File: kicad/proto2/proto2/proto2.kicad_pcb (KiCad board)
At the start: 2 copper layers, 100 x 100 mm, 0 parts

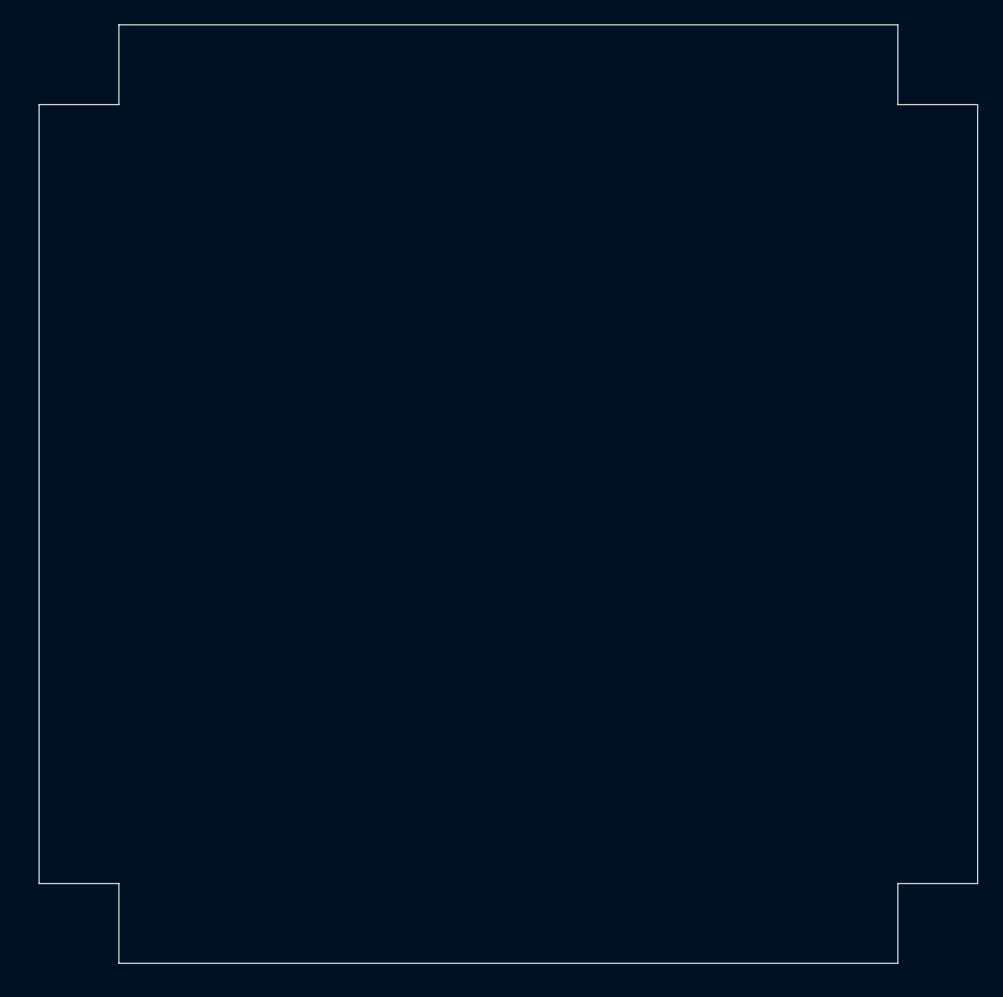
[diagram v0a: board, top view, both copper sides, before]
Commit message: pdf et png proto2
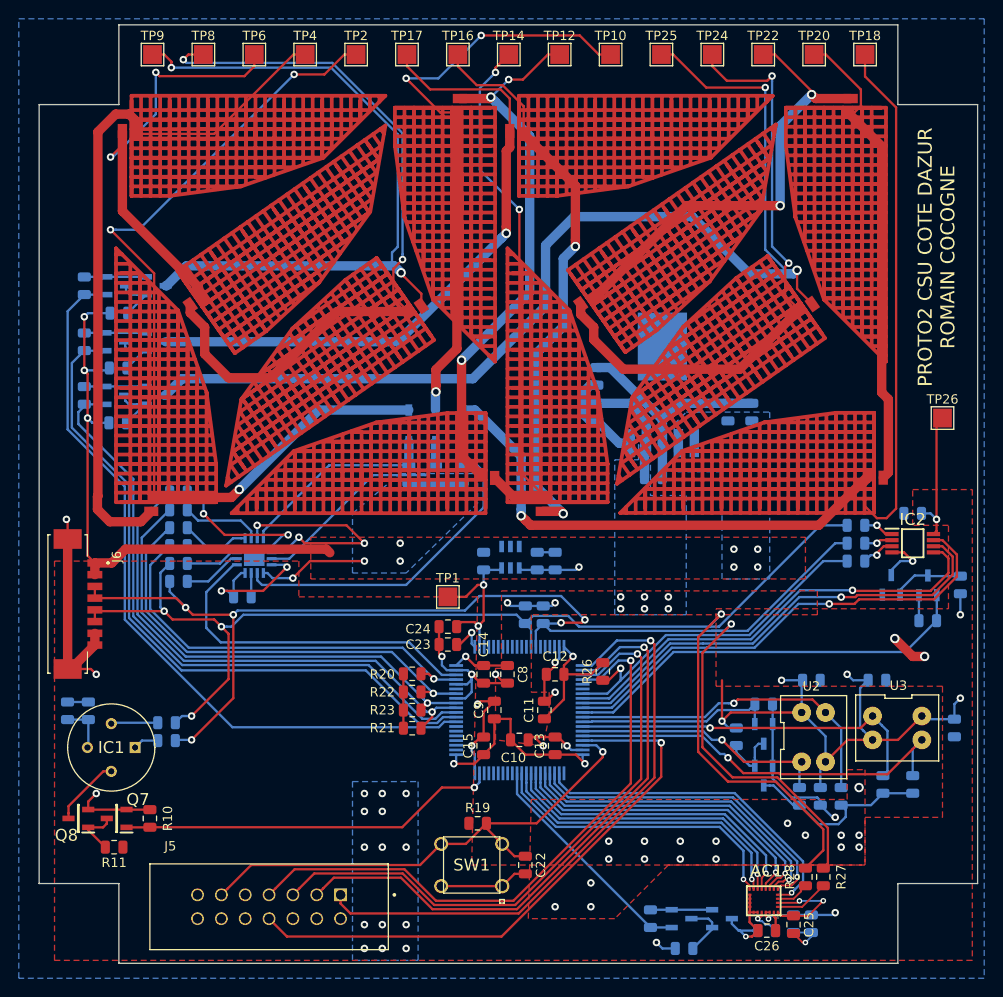
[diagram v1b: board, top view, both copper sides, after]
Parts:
- added AC1: LSM9DS1TR, panneaux_solaires:LGA-24L_3X3.5X1MM_, F.Cu at (168.3, 144.8)
- added C1: 100nF, Capacitor_SMD:C_0805_2012Metric, B.Cu at (144.1, 108.6)
- added C10: 10uF, Capacitor_SMD:C_0805_2012Metric, F.Cu at (142.2, 127.6)
- added C11: 10uF, Capacitor_SMD:C_0805_2012Metric, F.Cu at (144.9, 124.5)
- added C12: 10nF, Capacitor_SMD:C_0805_2012Metric, F.Cu at (146.1, 120.7)
- added C13: 10nF, Capacitor_SMD:C_0805_2012Metric, F.Cu at (146.1, 128.3)
- added C14: 10nF, Capacitor_SMD:C_0805_2012Metric, F.Cu at (138.4, 120.7)
- added C15: 10nF, Capacitor_SMD:C_0805_2012Metric, F.Cu at (138.4, 128.3)
- added C2: 1uF, Capacitor_SMD:C_0805_2012Metric, B.Cu at (146.1, 108.6)
- added C22: 2.2nF, Capacitor_SMD:C_0805_2012Metric, F.Cu at (142.9, 141.0)
- added C23: 100nF, Capacitor_SMD:C_0805_2012Metric, F.Cu at (134.6, 115.6)
- added C24: 100nF, Capacitor_SMD:C_0805_2012Metric, F.Cu at (134.6, 117.5)
- added C25: 100nF, Capacitor_SMD:C_0805_2012Metric, F.Cu at (171.4, 147.3)
- added C26: 100nF, Capacitor_SMD:C_0805_2012Metric, F.Cu at (168.6, 148.0)
- added C27: 10nF, Capacitor_SMD:C_0805_2012Metric, B.Cu at (168.6, 148.0)
- added C28: 100nF, Capacitor_SMD:C_0805_2012Metric, B.Cu at (173.4, 147.2)
- added C29: 10uF, Capacitor_SMD:C_0805_2012Metric, B.Cu at (171.4, 147.2)
- added C3: 1uF, Capacitor_SMD:C_0805_2012Metric, B.Cu at (138.4, 108.6)
- added C30: 100nF, Capacitor_SMD:C_0805_2012Metric, B.Cu at (174.3, 133.7)
- added C31: 100nF, Capacitor_SMD:C_0805_2012Metric, B.Cu at (180.3, 121.3)
- added C32: 100nF, Capacitor_SMD:C_0805_2012Metric, B.Cu at (188.6, 126.4)
- added C33: 100nF, Capacitor_SMD:C_0805_2012Metric, B.Cu at (173.4, 121.3)
- added C34: 100nF, Capacitor_SMD:C_0805_2012Metric, B.Cu at (164.5, 92.7)
- added C35: 2.2uF, Capacitor_SMD:C_0805_2012Metric, B.Cu at (167.0, 92.7)
- added C36: 47nF, Capacitor_SMD:C_0805_2012Metric, B.Cu at (156.5, 99.7)
- added C37: 100nF, Capacitor_SMD:C_0805_2012Metric, B.Cu at (112.7, 112.4)
- added C4: 10uF, Capacitor_SMD:C_0805_2012Metric, B.Cu at (96.3, 124.5)
- added C5: 100nF, Capacitor_SMD:C_0805_2012Metric, B.Cu at (94.1, 124.5)
- added C7: 100nF, Capacitor_SMD:C_0805_2012Metric, B.Cu at (184.2, 103.5)
- added C8: 10uF, Capacitor_SMD:C_0805_2012Metric, F.Cu at (141.0, 120.7)
- added C9: 10uF, Capacitor_SMD:C_0805_2012Metric, F.Cu at (139.6, 124.5)
- added D1: D_Schottky, panneaux_solaires:SOD3715X135N, B.Cu at (130.5, 94.2)
- added D2: D_Schottky, panneaux_solaires:SOD3715X135N, B.Cu at (133.3, 94.2)
- added D3: D_Schottky, panneaux_solaires:SOD3715X135N, B.Cu at (136.1, 94.2)
- added IC1: MLX90641ESF-BAA-000-TU, panneaux_solaires:MLX90621ESFBAB000SP, F.Cu at (101.3, 128.4)
- added IC2: PCT2075DP,118, panneaux_solaires:SOP65P490X110-8N, F.Cu at (184.2, 106.7)
- added IC3: MSP430FR5964IPNR, panneaux_solaires:QFP50P1400X1400X160-80N, B.Cu at (142.2, 124.5)
- added J5: HEADER_2x7_2.54MM, panneaux_solaires:TE_5104338-2, F.Cu at (123.2, 144.1)
- added J6: 0532610871, panneaux_solaires:MOLEX_0532610871, F.Cu at (94.1, 113.2)
- added Q1: RUR040N02HZGTL, panneaux_solaires:RUR040N02HZGTL, B.Cu at (99.3, 79.2)
- added Q10: RUR040N02HZGTL, panneaux_solaires:RUR040N02HZGTL, B.Cu at (181.9, 111.1)
- added Q11: RUR040N02HZGTL, panneaux_solaires:RUR040N02HZGTL, B.Cu at (159.5, 146.7)
- added Q12: RUR040N02HZGTL, panneaux_solaires:RUR040N02HZGTL, B.Cu at (163.8, 146.7)
- added Q13: RUR040N02HZGTL, panneaux_solaires:RUR040N02HZGTL, B.Cu at (168.3, 127.0)
- added Q14: RUR040N02HZGTL, panneaux_solaires:RUR040N02HZGTL, B.Cu at (168.3, 131.4)
- added Q2: RUR040N02HZGTL, panneaux_solaires:RUR040N02HZGTL, B.Cu at (103.5, 79.2)
- added Q3: RUR040N02HZGTL, panneaux_solaires:RUR040N02HZGTL, B.Cu at (99.2, 85.2)
- added Q4: RUR040N02HZGTL, panneaux_solaires:RUR040N02HZGTL, B.Cu at (103.5, 85.2)
- added Q5: RUR040N02HZGTL, panneaux_solaires:RUR040N02HZGTL, B.Cu at (99.2, 90.9)
- added Q6: RUR040N02HZGTL, panneaux_solaires:RUR040N02HZGTL, B.Cu at (103.5, 90.9)
- added Q7: RUR040N02HZGTL, panneaux_solaires:RUR040N02HZGTL, F.Cu at (99.3, 136.0)
- added Q8: RUR040N02HZGTL, panneaux_solaires:RUR040N02HZGTL, F.Cu at (95.2, 136.0)
- added Q9: RUR040N02HZGTL, panneaux_solaires:RUR040N02HZGTL, B.Cu at (185.8, 111.2)
- added R1: 20R, Resistor_SMD:R_0805_2012Metric, B.Cu at (95.9, 79.2)
- added R10: 20R, Resistor_SMD:R_0805_2012Metric, F.Cu at (102.9, 136.0)
- added R11: 1M, Resistor_SMD:R_0805_2012Metric, F.Cu at (99.1, 139.1)
- added R12: 330R, Resistor_SMD:R_0805_2012Metric, B.Cu at (104.6, 125.8)
- added R13: 330R, Resistor_SMD:R_0805_2012Metric, B.Cu at (104.6, 127.7)
- added R14: 20R, Resistor_SMD:R_0805_2012Metric, B.Cu at (185.8, 114.9)
- added R15: 1M, Resistor_SMD:R_0805_2012Metric, B.Cu at (189.2, 111.1)
- added R16: 330R, Resistor_SMD:R_0805_2012Metric, B.Cu at (178.1, 104.8)
- added R17: 330R, Resistor_SMD:R_0805_2012Metric, B.Cu at (178.1, 106.7)
- added R18: 330R, Resistor_SMD:R_0805_2012Metric, B.Cu at (178.1, 108.6)
- added R19: 47kR, Resistor_SMD:R_0805_2012Metric, F.Cu at (137.8, 136.5)
- added R2: 1M, Resistor_SMD:R_0805_2012Metric, B.Cu at (99.6, 82.2)
- added R20: 10k, Resistor_SMD:R_0805_2012Metric, F.Cu at (130.8, 120.6)
- added R21: 10k, Resistor_SMD:R_0805_2012Metric, F.Cu at (130.8, 126.4)
- added R22: 10k, Resistor_SMD:R_0805_2012Metric, F.Cu at (130.8, 122.5)
- added R23: 10k, Resistor_SMD:R_0805_2012Metric, F.Cu at (130.8, 124.5)
- added R24: 10k, Resistor_SMD:R_0805_2012Metric, B.Cu at (142.9, 114.3)
- added R25: 10k, Resistor_SMD:R_0805_2012Metric, B.Cu at (144.8, 114.3)
- added R26: 10k, Resistor_SMD:R_0805_2012Metric, F.Cu at (151.1, 120.3)
- added R27: 330R, Resistor_SMD:R_0805_2012Metric, F.Cu at (174.6, 142.2)
- added R28: 330R, Resistor_SMD:R_0805_2012Metric, F.Cu at (172.7, 142.2)
- added R29: 20R, Resistor_SMD:R_0805_2012Metric, B.Cu at (156.2, 146.7)
- added R3: 100mR, Resistor_SMD:R_0805_2012Metric, B.Cu at (130.5, 99.3)
- added R30: 1M, Resistor_SMD:R_0805_2012Metric, B.Cu at (159.8, 149.9)
- added R31: 20R, Resistor_SMD:R_0805_2012Metric, B.Cu at (168.3, 123.8)
- added R32: 1M, Resistor_SMD:R_0805_2012Metric, B.Cu at (165.4, 127.3)
- added R33: 10k, Resistor_SMD:R_0805_2012Metric, B.Cu at (172.1, 133.7)
- added R34: 10k, Resistor_SMD:R_0805_2012Metric, B.Cu at (176.5, 133.7)
- added R35: 10k, Resistor_SMD:R_0805_2012Metric, B.Cu at (181.0, 132.4)
- added R36: 10k, Resistor_SMD:R_0805_2012Metric, B.Cu at (184.2, 132.4)
- added R37: 3.3k, Resistor_SMD:R_0805_2012Metric, B.Cu at (150.5, 92.7)
- added R38: 2k, Resistor_SMD:R_0805_2012Metric, B.Cu at (150.5, 88.9)
- added R39: 330R, Resistor_SMD:R_0805_2012Metric, B.Cu at (105.9, 110.7)
- added R4: 20R, Resistor_SMD:R_0805_2012Metric, B.Cu at (95.9, 85.2)
- added R40: 330R, Resistor_SMD:R_0805_2012Metric, B.Cu at (105.9, 108.8)
- added R41: 330R, Resistor_SMD:R_0805_2012Metric, B.Cu at (105.9, 106.9)
- added R42: 330R, Resistor_SMD:R_0805_2012Metric, B.Cu at (105.9, 101.2)
- added R43: 330R, Resistor_SMD:R_0805_2012Metric, B.Cu at (105.9, 105.0)
- added R44: 330R, Resistor_SMD:R_0805_2012Metric, B.Cu at (105.9, 103.1)
- added R5: 1M, Resistor_SMD:R_0805_2012Metric, B.Cu at (99.5, 88.0)
- added R6: 100mR, Resistor_SMD:R_0805_2012Metric, B.Cu at (133.3, 99.3)
- added R7: 20R, Resistor_SMD:R_0805_2012Metric, B.Cu at (95.9, 90.9)
- added R8: 1M, Resistor_SMD:R_0805_2012Metric, B.Cu at (99.4, 93.9)
- added R9: 100mR, Resistor_SMD:R_0805_2012Metric, B.Cu at (136.1, 99.3)
- added SC1: Solar_Cell, panneaux_solaires:TRISOLX-T01, F.Cu at (99.5, 102.2)
- added SC10: Solar_Cell, panneaux_solaires:TRISOLX-T01, F.Cu at (181.1, 60.4)
- added SC11: Solar_Cell, panneaux_solaires:TRISOLX-T01, F.Cu at (147.7, 77.7)
- added SC12: Solar_Cell, panneaux_solaires:TRISOLX-T01, F.Cu at (174.6, 84.7)
- added SC2: Solar_Cell, panneaux_solaires:TRISOLX-T01, F.Cu at (101.0, 59.3)
- added SC3: Solar_Cell, panneaux_solaires:TRISOLX-T01, F.Cu at (106.1, 77.8)
- added SC4: Solar_Cell, panneaux_solaires:TRISOLX-T01, F.Cu at (132.9, 84.9)
- added SC5: Solar_Cell, panneaux_solaires:TRISOLX-T01, F.Cu at (139.4, 60.4)
- added SC6: Solar_Cell, panneaux_solaires:TRISOLX-T01, F.Cu at (138.5, 103.2)
- added SC7: Solar_Cell, panneaux_solaires:TRISOLX-T01, F.Cu at (141.2, 102.2)
- added SC8: Solar_Cell, panneaux_solaires:TRISOLX-T01, F.Cu at (142.3, 59.3)
- added SC9: Solar_Cell, panneaux_solaires:TRISOLX-T01, F.Cu at (179.9, 103.2)
- added SW1: BP_DROIT_TRAV-switch, panneaux_solaires:switch_fsm6jh_tyco, F.Cu at (137.2, 141.0)
- added TP1: TestPoint, panneaux_solaires:TestPoint_Pad_2.0x2.0mm, F.Cu at (134.6, 112.4)
- added TP10: TestPoint, panneaux_solaires:TestPoint_Pad_2.0x2.0mm, F.Cu at (152.0, 54.6)
- added TP12: TestPoint, panneaux_solaires:TestPoint_Pad_2.0x2.0mm, F.Cu at (146.5, 54.6)
- added TP14: TestPoint, panneaux_solaires:TestPoint_Pad_2.0x2.0mm, F.Cu at (141.1, 54.6)
- added TP16: TestPoint, panneaux_solaires:TestPoint_Pad_2.0x2.0mm, F.Cu at (135.7, 54.6)
- added TP17: TestPoint, panneaux_solaires:TestPoint_Pad_2.0x2.0mm, F.Cu at (130.3, 54.6)
- added TP18: TestPoint, panneaux_solaires:TestPoint_Pad_2.0x2.0mm, F.Cu at (179.1, 54.6)
- added TP2: TestPoint, panneaux_solaires:TestPoint_Pad_2.0x2.0mm, F.Cu at (124.8, 54.6)
- added TP20: TestPoint, panneaux_solaires:TestPoint_Pad_2.0x2.0mm, F.Cu at (173.6, 54.6)
- added TP22: TestPoint, panneaux_solaires:TestPoint_Pad_2.0x2.0mm, F.Cu at (168.2, 54.6)
- added TP24: TestPoint, panneaux_solaires:TestPoint_Pad_2.0x2.0mm, F.Cu at (162.8, 54.6)
- added TP25: TestPoint, panneaux_solaires:TestPoint_Pad_2.0x2.0mm, F.Cu at (157.4, 54.6)
- added TP26: TestPoint, panneaux_solaires:TestPoint_Pad_2.0x2.0mm, F.Cu at (187.3, 93.3)
- added TP4: TestPoint, panneaux_solaires:TestPoint_Pad_2.0x2.0mm, F.Cu at (119.4, 54.6)
- added TP6: TestPoint, panneaux_solaires:TestPoint_Pad_2.0x2.0mm, F.Cu at (114.0, 54.6)
- added TP8: TestPoint, panneaux_solaires:TestPoint_Pad_2.0x2.0mm, F.Cu at (108.6, 54.6)
- added TP9: TestPoint, panneaux_solaires:TestPoint_Pad_2.0x2.0mm, F.Cu at (103.1, 54.6)
- added U1: LT1790ACS6-1.25TRMPBF, panneaux_solaires:SOT95P280X100-6N, B.Cu at (141.3, 108.2)
- added U2: S3274-05, panneaux_solaires:S3274-05, F.Cu at (174.2, 116.2)
- added U3: S3274-05, panneaux_solaires:S3274-05, F.Cu at (193.7, 127.0)
- added U4: NCP59302DSADJR4G, panneaux_solaires:NCP59302DSADJR4G, B.Cu at (157.5, 89.8)
- added U5: INA3221AIRGVR, panneaux_solaires:QFN65P400X400X100-17N, B.Cu at (114.0, 108.0)
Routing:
- net JTAG_VCC-TARGET: track 0.00 -> 182.5 mm, vias 0 -> 39
- net UC19: track 0.00 -> 176.6 mm, vias 0 -> 34
- net SCL: track 0.00 -> 158.7 mm, vias 0 -> 6
- net SDA: track 0.00 -> 149.5 mm, vias 0 -> 4
- net Net-(Q6-Pad2): track 0.00 -> 120.1 mm, vias 0 -> 2
- net VOLTMETER3: track 0.00 -> 112.0 mm, vias 0 -> 1
- net AMPERMETER-: track 0.00 -> 110.3 mm, vias 0 -> 15
- net VOLTMETER1: track 0.00 -> 95.3 mm, vias 0 -> 3
- net Net-(SC3-Pad2): track 0.00 -> 80.5 mm, vias 0 -> 2
- net BNK1_CONTROL: track 0.00 -> 80.5 mm
- net Net-(Q2-Pad2): track 0.00 -> 76.1 mm, vias 0 -> 2
- net Net-(SC1-Pad2): track 0.00 -> 75.0 mm
- net BNK2_CONTROL: track 0.00 -> 73.6 mm
- net Net-(Q4-Pad2): track 0.00 -> 69.2 mm, vias 0 -> 1
- net BNK3_CONTROL: track 0.00 -> 66.7 mm
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- added copper zone on B.Cu, net AMPERMETER-
- added copper zone on F.Cu, net AMPERMETER-
- added copper zone on B.Cu, net JTAG_VCC-TARGET
- added copper zone on F.Cu, net JTAG_VCC-TARGET
- added copper zone on B.Cu, net UC19
- added copper zone on F.Cu, net UC19
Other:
- board text added: "PROTO2 CSU COTE DAZUR ROMAIN COCOGNE"
